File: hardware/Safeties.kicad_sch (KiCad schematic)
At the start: 19 parts, among them K1 6-1419128-4, Q1 2N7002, Q2 2N7002, Q3 2N7002, U2 74LVC1G86, U3 74AUP1G32

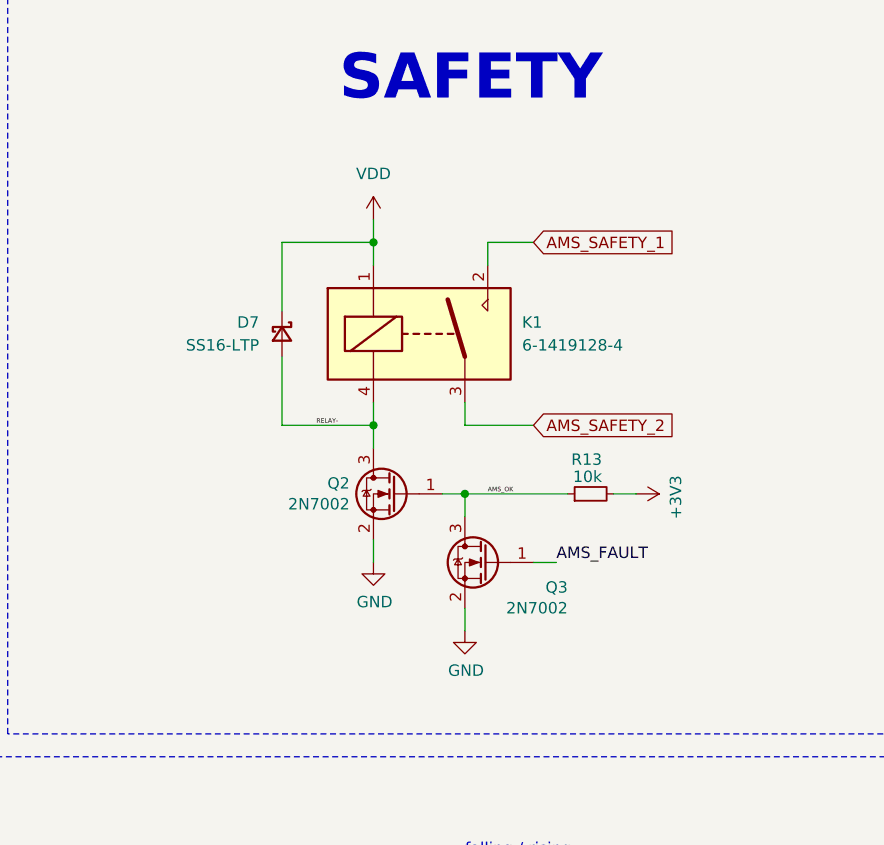
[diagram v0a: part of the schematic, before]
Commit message: changes tbc
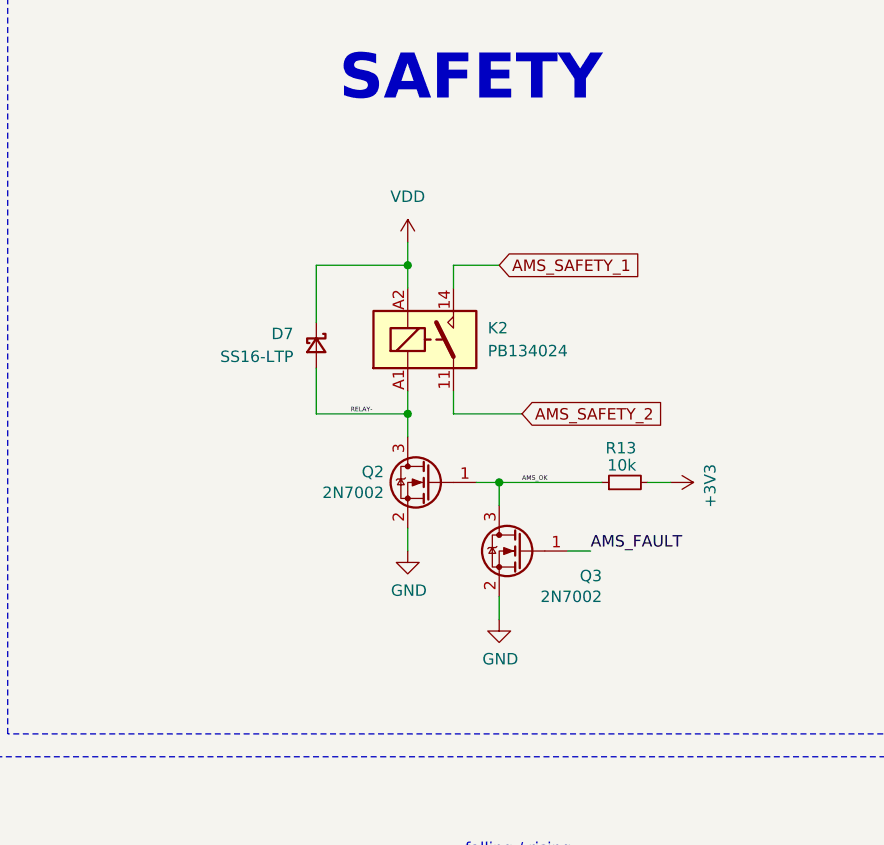
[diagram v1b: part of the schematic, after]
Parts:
- removed K1: 6-1419128-4, 614191284, symbol 6-1419128-4:6-1419128-4
- added K2: PB134024, Samacsys:PB134024, symbol Samacsys_kicad_sym:PB134024
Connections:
- net AMS_SAFETY_1: now also K2.14 (NO)
- net AMS_SAFETY_2: now also K2.11 (COM)
- net RELAY-: now also K2.A1 (COIL_1)
- net VDD: now also K2.A2 (COIL_2)
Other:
- moved on the sheet: D7, Q2, Q3, R13
